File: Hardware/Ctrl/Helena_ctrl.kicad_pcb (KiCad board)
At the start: 2 copper layers, 38 x 18 mm, 41 parts, among them P1 CONN_01X06, P2 CONN_01X04, Q1 BC857C, SW1 SW_PUSH, U1 antenna-gnd, U2 nrf51822-qfax, U3 MPU-6050, Y1 16MHz

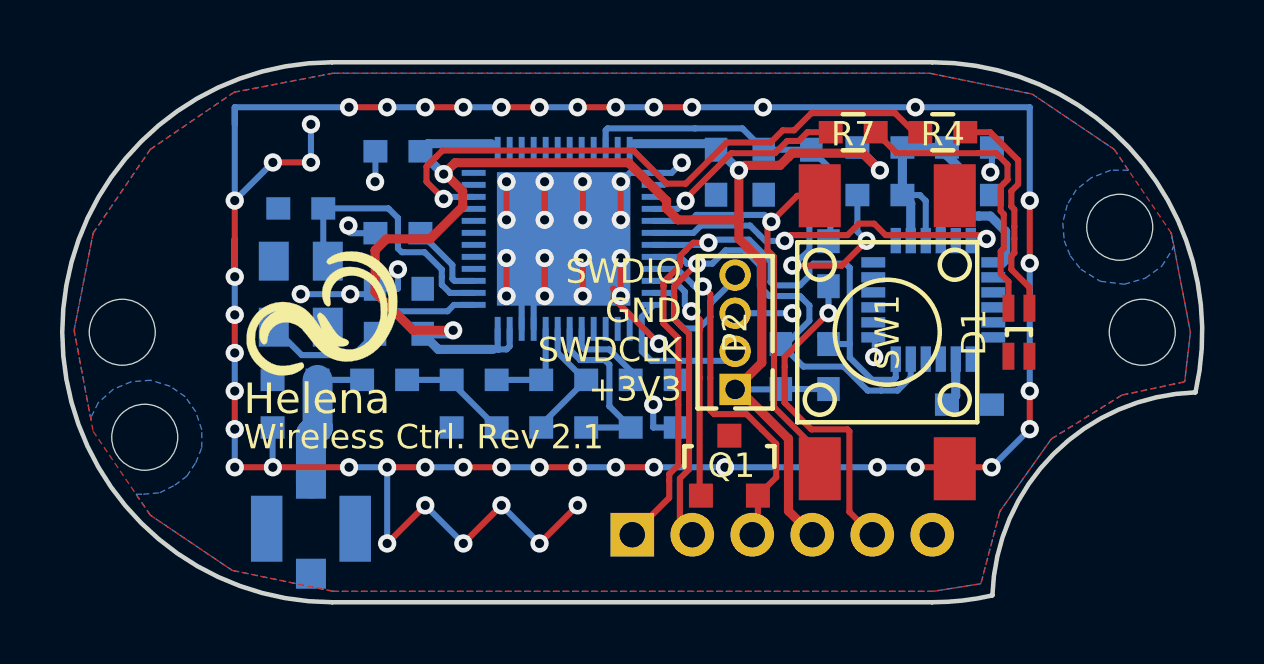
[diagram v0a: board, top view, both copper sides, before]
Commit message: updated control board
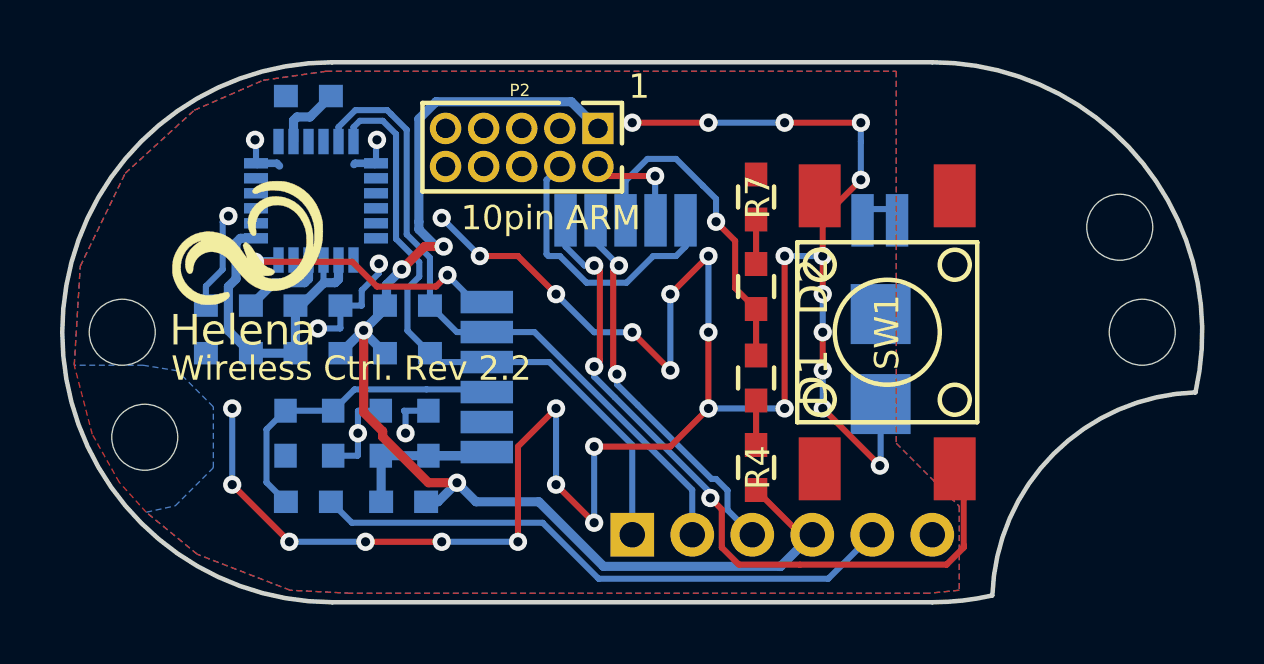
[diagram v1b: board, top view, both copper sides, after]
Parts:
- removed C10, C7: 22p, rt_device:C_0603_THERMaL_RELIEF
- removed C11, C12, C3, C4: 100n, rt_device:C_0603_THERMaL_RELIEF
- removed C5: 1p0, rt_device:C_0603_THERMaL_RELIEF
- removed C6: 1n, rt_device:C_0603_THERMaL_RELIEF
- removed C8: 2p2, rt_device:C_0603_THERMaL_RELIEF
- removed C9: 2n2, rt_device:C_0603_THERMaL_RELIEF
- removed L1: 3n3, rt_device:C_0603_THERMaL_RELIEF
- removed L2: 4n7, rt_device:C_0603_THERMaL_RELIEF
- removed L3: 10n, rt_device:C_0603_THERMaL_RELIEF
- removed Q1: BC857C, TO_SOT_Packages_SMD:SOT-23
- removed U1: antenna-gnd, rt_antennas:MML_R302.302.000
- removed Y1: 16MHz, rt_XTAL:XTAL_MT_3.2mm_x_2.5mm
- added D2: LED_BLUE, rt_device:C_0603_THERMaL_RELIEF, F.Cu at (54.1, 148.5)
- added FB2: FB, rt_device:C_0603_THERMaL_RELIEF, B.Cu at (42.4, 155.7)
- C1: value dnp -> 2u2/16
- C2: value 1p5 -> 100n
- D1: value Double_LED -> LED_RED; footprint rt_leds:Duo-Led_0603 -> rt_device:C_0603_THERMaL_RELIEF
- P2: value CONN_01X04 -> CONN_02X05; footprint rt_Pin_Header:Pin_Header_Straight_1x04_Pitch1.27mm -> rt_Pin_Header:Pin_Header_Straight_2x05_Pitch1.27mm
- U2: value nrf51822-qfax -> nrf51822-04AT_Module; footprint Housings_DFN_QFN:UQFN-48-1EP_6x6mm_Pitch0.4mm -> WT51822-S4AT
- moved C13 25.6 mm to (36.5, 150.7), turned to 180 degrees
- moved C15 25.0 mm to (36.5, 149.1), turned to 180 degrees
- moved C17 24.3 mm to (39.2, 142.1), turned to 180 degrees
- moved U3 20.8 mm to (39.5, 145.6), turned to 180 degrees
- moved FB1 19.9 mm to (39.5, 150.7), turned to 180 degrees
- moved R2 19.6 mm to (38.4, 153.4)
- moved C14 19.1 mm to (39.5, 149.1), turned to 0 degrees
- moved R1 19.1 mm to (39.2, 155.7), turned to 180 degrees
- moved C16 16.8 mm to (40.0, 153.4)
- moved R3 14.0 mm to (42.5, 150.7), turned to 0 degrees
- moved R4 12.8 mm to (54.1, 154.5), turned to 90 degrees
- moved R5 12.6 mm to (42.5, 149.1), turned to 0 degrees
- moved U2 11.7 mm to (58.8, 150.4), turned to 90 degrees
- moved P2 9.83 mm to (48.9, 143.2), turned to 270 degrees
- moved D1 8.89 mm to (54.1, 151.5), turned to 270 degrees
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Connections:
- D1 pad 1: GND -> /~LED_RED~/LED_BLUE
- P2 pad 2: /SWDCLK -> /SWDIO
- P2 pad 4: /SWDIO -> /SWDCLK
- R4 pad 1: /LED_RED -> +3V3
- R4 pad 2: Net-(D1-Pad4) -> Net-(D1-Pad2)
- R7 pad 1: /LED_BLUE -> Net-(D2-Pad1)
- R7 pad 2: Net-(D1-Pad2) -> GND
- U2 pad 1: +3V3 -> Net-(C1-Pad1)
- U2 pad 10: /VIN_ADC -> /SWDIO
- U2 pad 11: Net-(U2-Pad11) -> /SWDCLK
- U2 pad 12: +3V3 -> GND
- U2 pad 15: Net-(U2-Pad15) -> GND
- U2 pad 2: Net-(U2-Pad2) -> GND
- U2 pad 3: Net-(U2-Pad3) -> /VIN_ADC
- U2 pad 4: Net-(U2-Pad4) -> /SDA
- U2 pad 5: Net-(U2-Pad5) -> /SCL
- U2 pad 6: Net-(U2-Pad6) -> /MPU_INT
- U2 pad 7: Net-(U2-Pad7) -> /BUTTON
- U2 pad 8: Net-(U2-Pad8) -> /BDEP_RX
- U2 pad 9: Net-(U2-Pad9) -> /~LED_RED~/LED_BLUE
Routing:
- net GND: track 159.0 -> 98.3 mm, vias 75 -> 39
- net /LED_RED: track 20.9 -> 0.00 mm, vias 1 -> 0
- net +3V3: track 57.5 -> 41.9 mm
- net /~LED_RED~/LED_BLUE: track 0.00 -> 11.0 mm, vias 0 -> 1
- net Net-(D1-Pad2): track 10.6 -> 1.48 mm
- net VPP: track 10.8 -> 19.7 mm, vias 1 -> 0
- net Net-(C10-Pad1): track 8.89 -> 0.00 mm
- net /BDEP_TX: track 8.40 -> 0.00 mm, vias 1 -> 0
- net /BUTTON: track 16.8 -> 25.1 mm, vias 1 -> 3
- net Net-(D1-Pad4): track 8.04 -> 0.00 mm
- net Net-(C7-Pad1): track 7.74 -> 0.00 mm
- net /LED_BLUE: track 7.06 -> 0.00 mm, vias 1 -> 0
- net Net-(C9-Pad1): track 6.09 -> 0.00 mm
- net /SDA: track 26.3 -> 20.9 mm, vias 1 -> 0
- net /SWDCLK: track 5.44 -> 10.0 mm
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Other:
- board text added: "1"
- board text added: "10pin ARM"
- board text added: "RT1703"
- board text added: "Wireless Ctrl. Rev 2.2"
- board text removed: "RT1612"
- board text removed: "SWDIO GND SWDCLK +3V3"
- board text removed: "Wireless Ctrl. Rev 2.1"
